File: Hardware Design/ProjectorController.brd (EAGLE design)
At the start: 46.7 x 38.1 mm, 18 parts, among them J1 5747844-4, J2 Cap Buttons, J3 Prog, J4 Prog/Run, J5 10118194-0001LF, U1 ESP-WROOM-32, U2 SP3232EEN-L

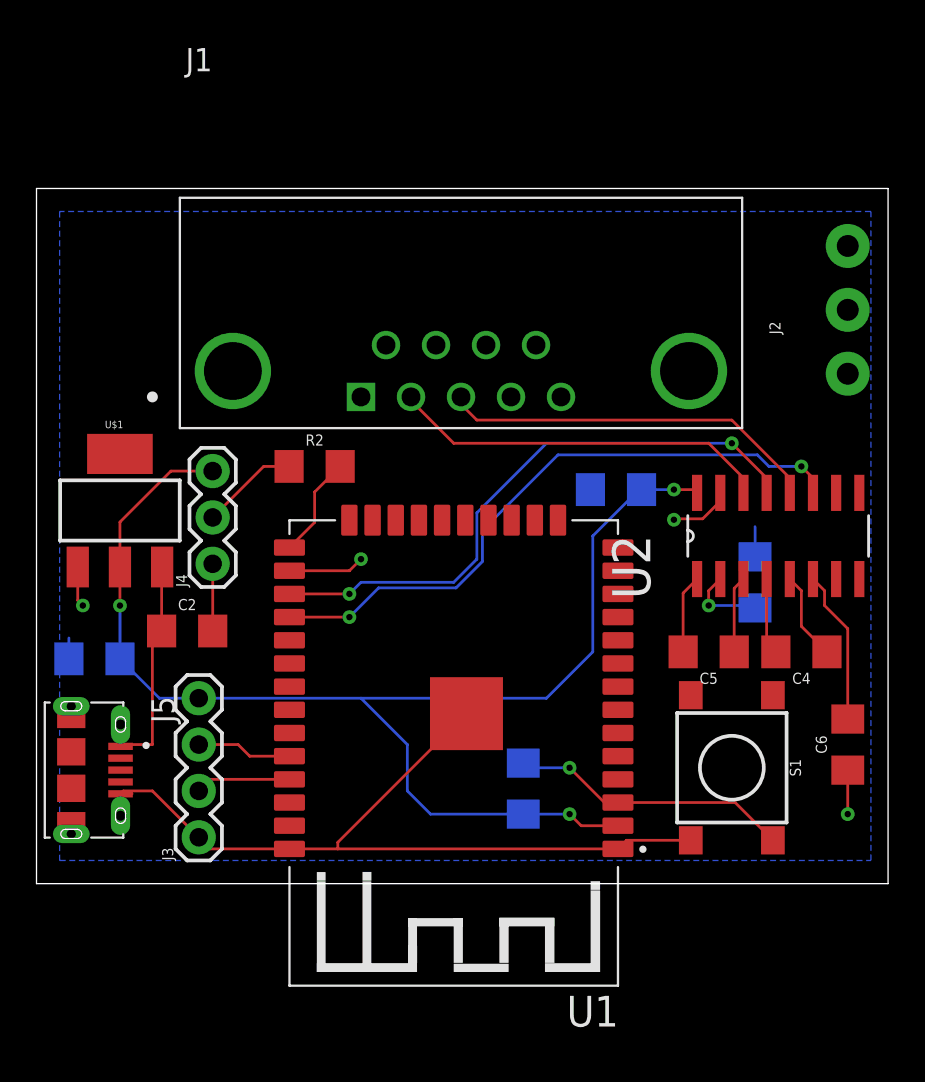
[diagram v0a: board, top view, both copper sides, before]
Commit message: Optimised Layout
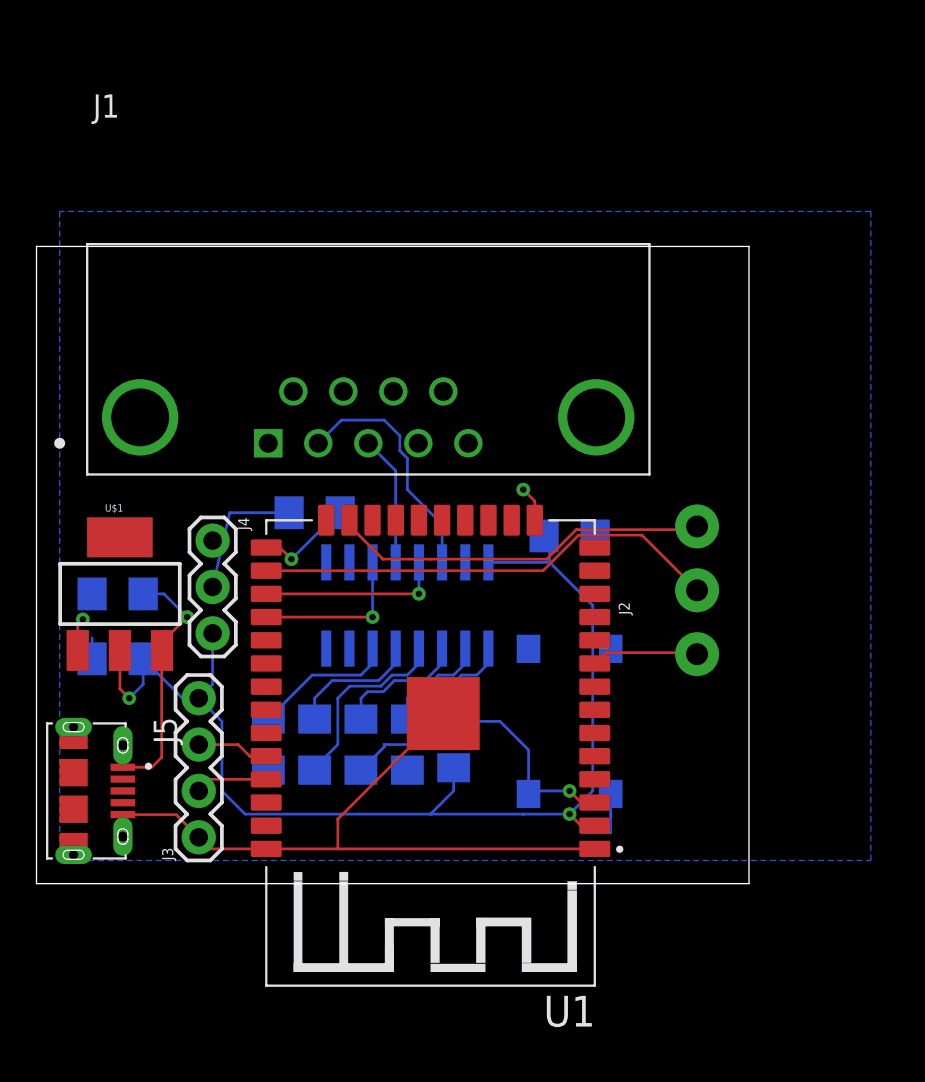
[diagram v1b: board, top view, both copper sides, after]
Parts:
- C1, C2: value (none) -> 10uF
- moved C6 31.7 mm to (16.5, 50.8), flipped to the bottom
- moved C4 27.1 mm to (19.1, 50.8), flipped to the bottom, turned to 270 degrees
- moved C7 21.0 mm to (24.1, 50.8), turned to 90 degrees
- moved U2 20.7 mm to (24.1, 58.4), flipped to the bottom
- moved C5 19.7 mm to (21.6, 50.8), flipped to the bottom, turned to 270 degrees
- moved J2 17.4 mm to (40.0, 55.8)
- moved S1 9.25 mm to (33.0, 52.1), flipped to the bottom
- moved J1 5.68 mm to (16.5, 67.3)
- moved R1 4.58 mm to (26.7, 50.9)
- moved U$1 4.57 mm to (8.38, 59.1)
- moved C2 4.32 mm to (8.26, 59.1), flipped to the bottom
- moved C3 3.59 mm to (33.0, 62.2), turned to 0 degrees
- moved R2 2.54 mm to (19.1, 63.5), flipped to the bottom, turned to 180 degrees
- moved U1 1.27 mm to (25.4, 53.3)
- moved C1 1.27 mm to (8.26, 55.5)
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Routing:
- net N$9: track 34.7 -> 9.28 mm, vias 2 -> 1
- net N$13: track 33.0 -> 10.1 mm, vias 2 -> 1
- net N$3: track 4.18 -> 25.7 mm, vias 1 -> 0
- net N$1: track 0.00 -> 21.0 mm
- net GND: track 60.1 -> 44.2 mm, vias 3 -> 2
- net N$11: track 20.9 -> 7.15 mm
- net 3V3: track 74.0 -> 63.9 mm, vias 3 -> 2
- net N$10: track 21.0 -> 13.2 mm
- net N$12: track 4.30 -> 11.9 mm
- net N$15: track 4.20 -> 10.5 mm
- net N$2: track 0.00 -> 5.88 mm
- net N$4: track 15.4 -> 11.2 mm
- net N$14: track 4.20 -> 7.19 mm
- net N$16: track 4.83 -> 7.19 mm
- net N$6: track 5.35 -> 7.42 mm
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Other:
- board size 46.7 x 38.1 mm -> 39 x 34.9 mm
